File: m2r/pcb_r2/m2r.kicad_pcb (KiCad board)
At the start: 2 copper layers, 56 x 56 mm, 105 parts, among them IC1 ADP3338, IC10 STM32F303C, IC2 ADP3335, IC3 ADuM1201, IC4 ADuM1201, IC5 ADuM1201, IC6 MTX2, IC8 MAX-7Q, P1 CONN_2, P2 SMA, P3 CONN_4, P4 CONN_4, P5 CONN_4, P6 SWD, P7 SMA, P8 CONN_2, P9 CONN_2, Q1 Q_PMOS_GSD_PSV, Q2 Q_NMOS_GSD_PSV, X10 8M, X11 M3 MOUNT, X12 M3 MOUNT, X13 M3 MOUNT, X14 M3 MOUNT

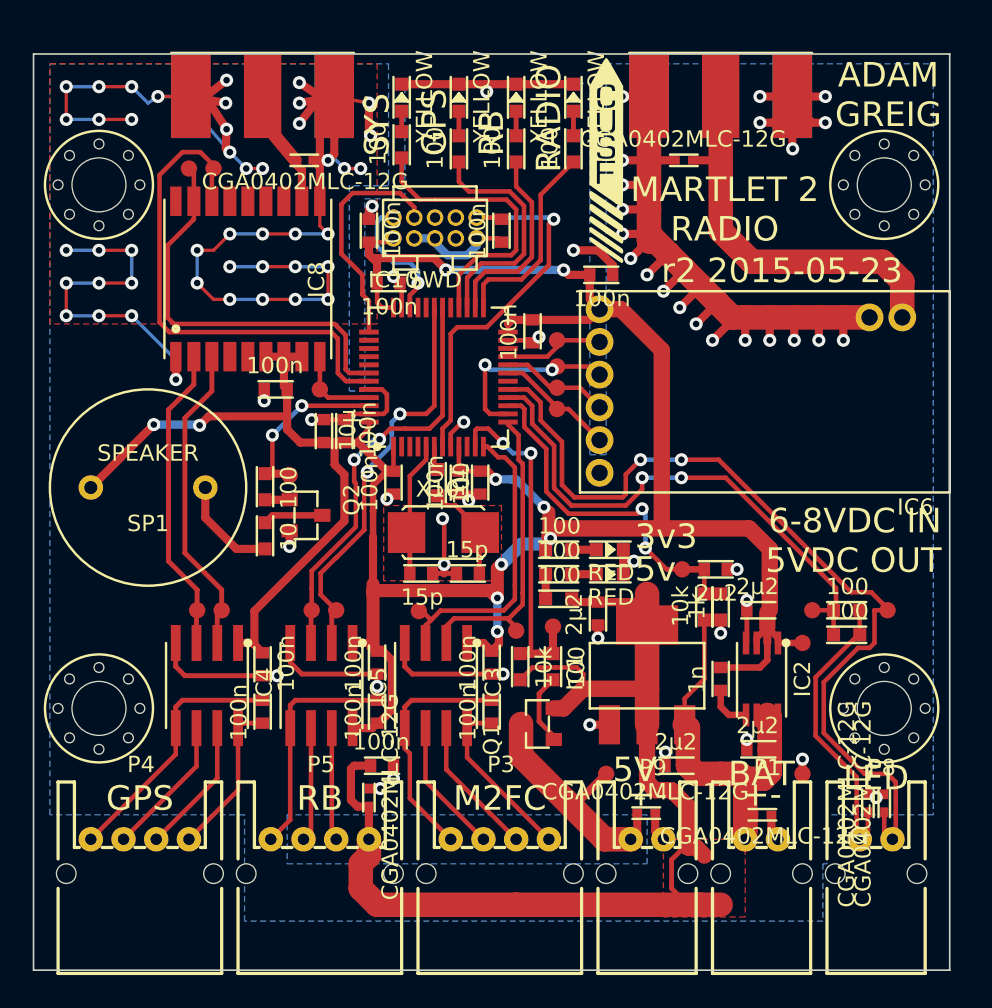
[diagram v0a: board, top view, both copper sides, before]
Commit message: routing updates
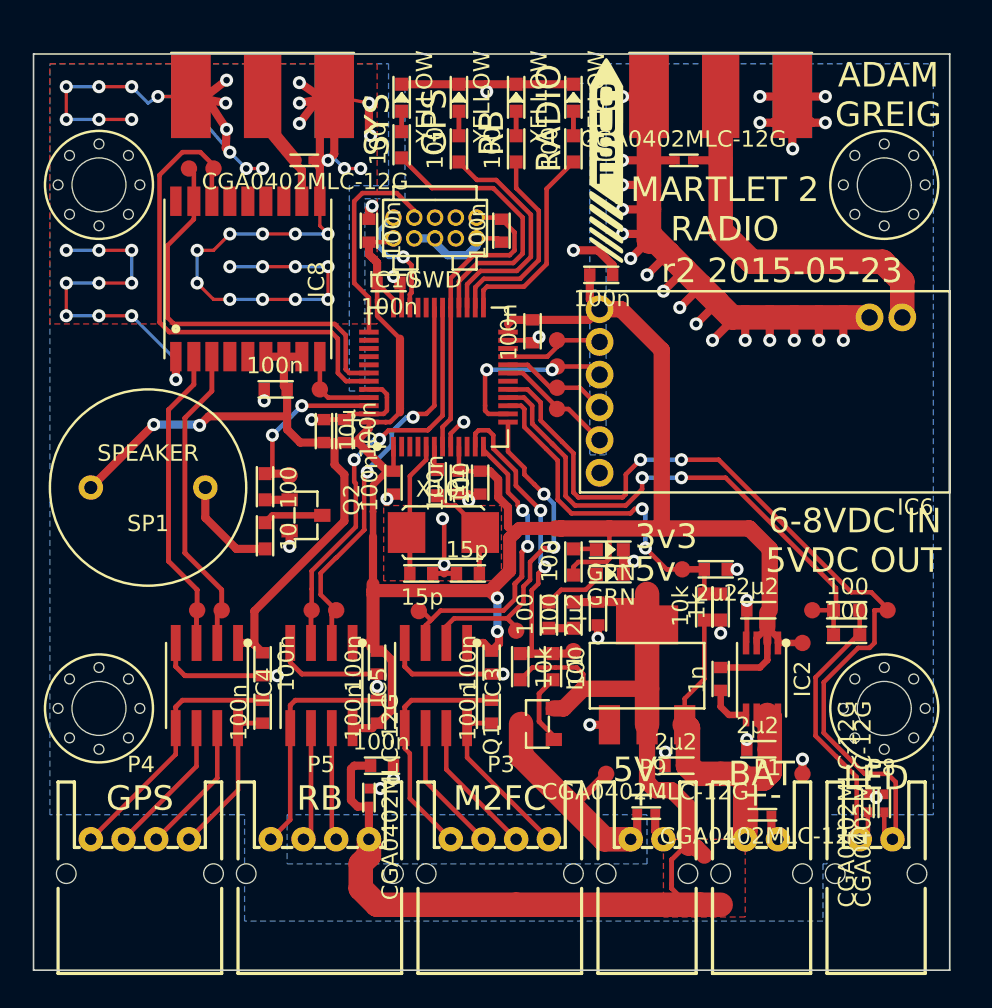
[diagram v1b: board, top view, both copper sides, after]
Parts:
- D1, D2: value RED -> GRN
- moved R7 2.20 mm to (109.5, 153.5), turned to 270 degrees
- moved TP27 1.95 mm to (111.0, 156.5)
- moved R9 0.22 mm to (111.0, 153.5), turned to 270 degrees
- moved R8 0.11 mm to (111.0, 150.2), turned to 270 degrees
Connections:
- IC10 pad 29: Net-(IC10-Pad29) -> nRST
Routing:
- net nRST: track 24.1 -> 18.9 mm, vias 1 -> 0
- net Net-(D2-Pad1): track 1.50 -> 3.78 mm
- net SER_IN: track 18.7 -> 20.6 mm, vias 0 -> 2
- net SWCLK: track 14.2 -> 13.1 mm
- net SWDIO: track 8.18 -> 7.33 mm
- net 5V_OUT: track 21.0 -> 20.5 mm
- net +3V3: track 172.0 -> 171.9 mm, vias 10 -> 4
- net SER_OUT: vias 0 -> 2
